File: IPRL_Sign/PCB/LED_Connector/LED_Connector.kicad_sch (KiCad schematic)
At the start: 2 parts, among them J1 Conn_01x02

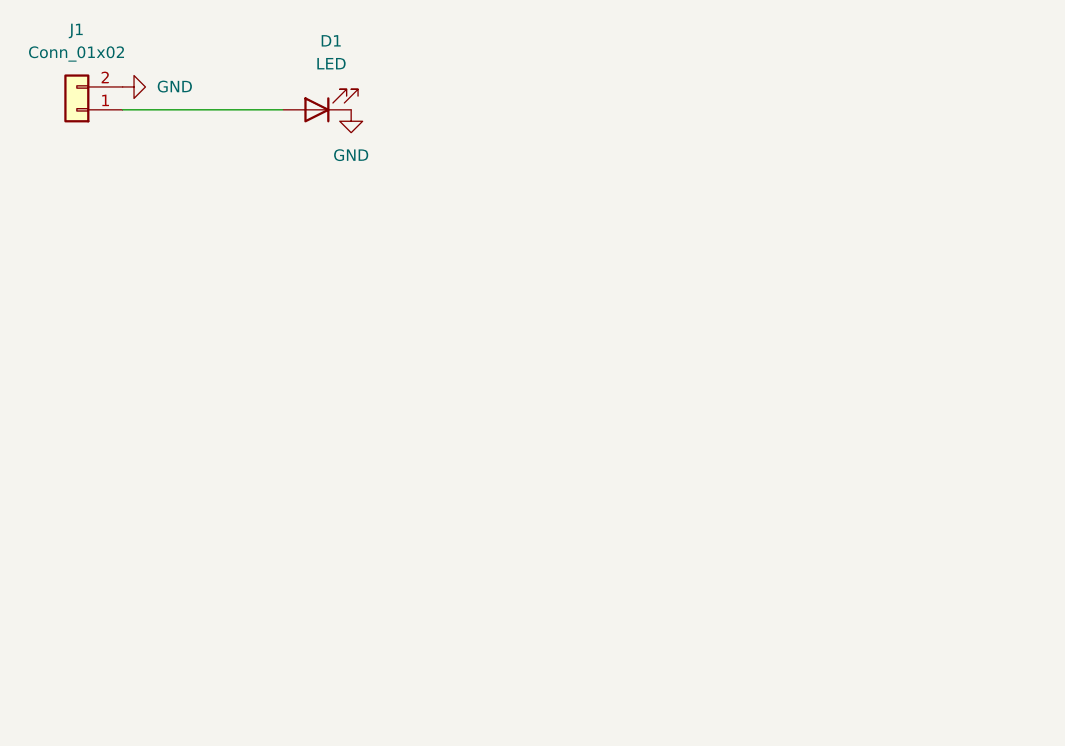
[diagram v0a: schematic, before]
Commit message: Added pdfs
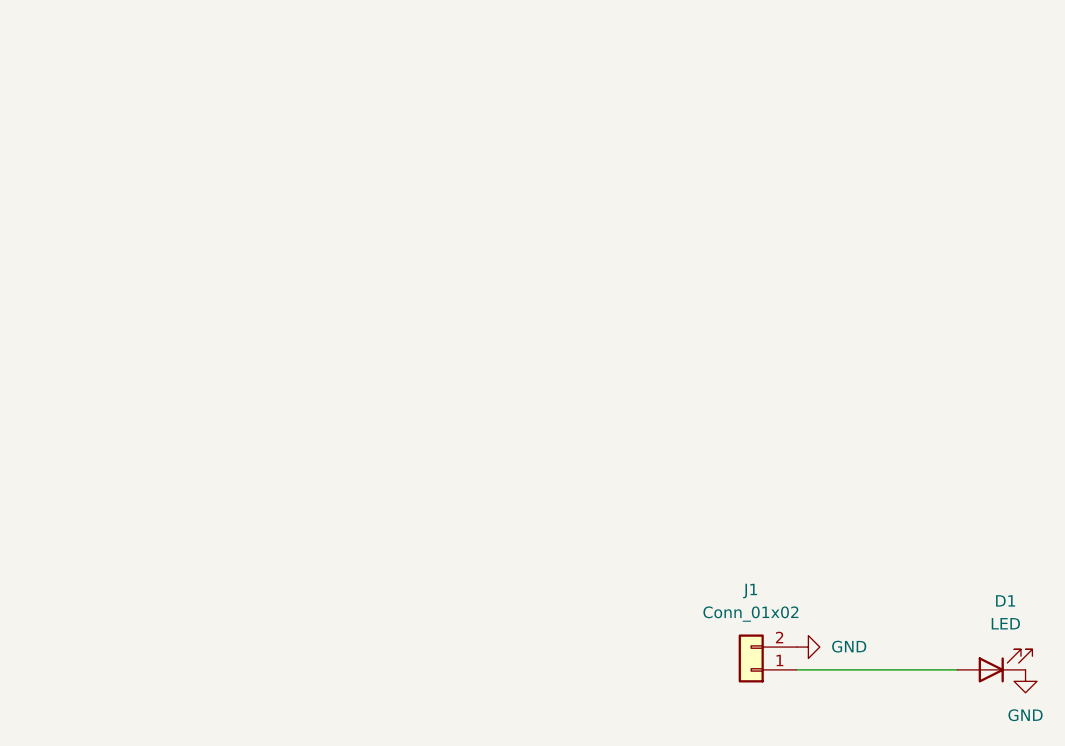
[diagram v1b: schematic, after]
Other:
- company: (none) -> Imperial Planetary Robotics Lab
- title: (none) -> IPRL Sign LED
- moved on the sheet: D1, J1
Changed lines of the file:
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@@
 	(generator_version "9.0")
 	(paper "A4")
+	(title_block
+		(title "IPRL Sign LED")
+		(date "2025-04-17")
+		(rev "1")
+		(company "Imperial Planetary Robotics Lab")
+	)
 	(wire
 		(pts
-			(xy 104.14 60.96) (xy 121.92 60.96)
+			(xy 179.07 123.19) (xy 196.85 123.19)
 		)
 		(stroke
@@
 	(symbol
 		(lib_id "power:GND")
-		(at 129.54 60.96 0)
+		(at 204.47 123.19 0)
 		(unit 1)
 		(exclude_from_sim no)
@@
 		(fields_autoplaced yes)
 		(property "Reference" "#PWR01"
-			(at 129.54 67.31 0)
+			(at 204.47 129.54 0)
 			(effects
 				(font
@@
 		)
 		(property "Value" "GND"
-			(at 129.54 66.04 0)
+			(at 204.47 128.27 0)
 			(effects
 				(font
@@
 		)
 		(property "Footprint" ""
-			(at 129.54 60.96 0)
+			(at 204.47 123.19 0)
 			(effects
 				(font
@@
 		)
 		(property "Datasheet" ""
-			(at 129.54 60.96 0)
+			(at 204.47 123.19 0)
 			(effects
 				(font
@@
 		)
 		(property "Description" "Power symbol creates a global label with name \"GND\" , ground"
-			(at 129.54 60.96 0)
+			(at 204.47 123.19 0)
 			(effects
 				(font
@@
 	(symbol
 		(lib_id "Connector_Generic:Conn_01x02")
-		(at 99.06 60.96 180)
+		(at 173.99 123.19 180)
 		(unit 1)
 		(exclude_from_sim no)
@@
 		(fields_autoplaced yes)
 		(property "Reference" "J1"
-			(at 99.06 52.07 0)
+			(at 173.99 114.3 0)
 			(effects
 				(font
@@
 		)
 		(property "Value" "Conn_01x02"
-			(at 99.06 54.61 0)
+			(at 173.99 116.84 0)
 			(effects
 				(font
@@
 		)
 		(property "Footprint" "Connector_Samtec_HPM_THT:Samtec_HPM-02-01-x-S_Straight_1x02_Pitch5.08mm"
-			(at 99.06 60.96 0)
+			(at 173.99 123.19 0)
 			(effects
 				(font
@@
 		)
 		(property "Datasheet" "~"
-			(at 99.06 60.96 0)
+			(at 173.99 123.19 0)
 			(effects
 				(font
@@
 		)
 		(property "Description" "Generic connector, single row, 01x02, script generated (kicad-library-utils/schlib/autogen/connector/)"
-			(at 99.06 60.96 0)
+			(at 173.99 123.19 0)
 			(effects
 				(font
@@
 	(symbol
 		(lib_id "power:GND")
-		(at 104.14 58.42 90)
+		(at 179.07 120.65 90)
 		(unit 1)
 		(exclude_from_sim no)
@@
 		(fields_autoplaced yes)
 		(property "Reference" "#PWR02"
-			(at 110.49 58.42 0)
+			(at 185.42 120.65 0)
 			(effects
 				(font
@@
 		)
 		(property "Value" "GND"
-			(at 107.95 58.4199 90)
+			(at 182.88 120.6499 90)
 			(effects
 				(font
@@
 		)
 		(property "Footprint" ""
-			(at 104.14 58.42 0)
+			(at 179.07 120.65 0)
 			(effects
 				(font
@@
 		)
 		(property "Datasheet" ""
-			(at 104.14 58.42 0)
+			(at 179.07 120.65 0)
 			(effects
 				(font
@@
 		)
 		(property "Description" "Power symbol creates a global label with name \"GND\" , ground"
-			(at 104.14 58.42 0)
+			(at 179.07 120.65 0)
 			(effects
 				(font
@@
 	(symbol
 		(lib_id "Device:LED")
-		(at 125.73 60.96 180)
+		(at 200.66 123.19 180)
 		(unit 1)
 		(exclude_from_sim no)
@@
 		(fields_autoplaced yes)
 		(property "Reference" "D1"
-			(at 127.3175 53.34 0)
+			(at 202.2475 115.57 0)
 			(effects
 				(font
@@
 		)
 		(property "Value" "LED"
-			(at 127.3175 55.88 0)
+			(at 202.2475 118.11 0)
 			(effects
 				(font
@@
 		)
 		(property "Footprint" "LED_THT:LED_D5.0mm"
-			(at 125.73 60.96 0)
+			(at 200.66 123.19 0)
 			(effects
 				(font
@@
 		)
 		(property "Datasheet" "~"
-			(at 125.73 60.96 0)
+			(at 200.66 123.19 0)
 			(effects
 				(font
@@
 		)
 		(property "Description" "Light emitting diode"
-			(at 125.73 60.96 0)
+			(at 200.66 123.19 0)
 			(effects
 				(font
@@
 		)
 		(property "Sim.Pins" "1=K 2=A"
-			(at 125.73 60.96 0)
-			(effects
-				(font
+			(at 200.66 123.19 0)
+			(effects
+				(font
